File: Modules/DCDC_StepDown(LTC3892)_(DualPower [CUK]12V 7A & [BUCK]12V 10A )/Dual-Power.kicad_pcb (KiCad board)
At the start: 4 copper layers, 58.4 x 55.9 mm, 81 parts, among them J1 Conn_02x05_Top_Bottom, J2 Conn_02x05_Top_Bottom, J3 Conn_01x02, Q1 BSC028N06LS3, Q2 BSC028N06LS3, Q3 BSC028N06LS3, Q4 BSC028N06LS3, Q5 BSC028N06LS3, U1 LTC3892EUHPBF, U2 LT1797

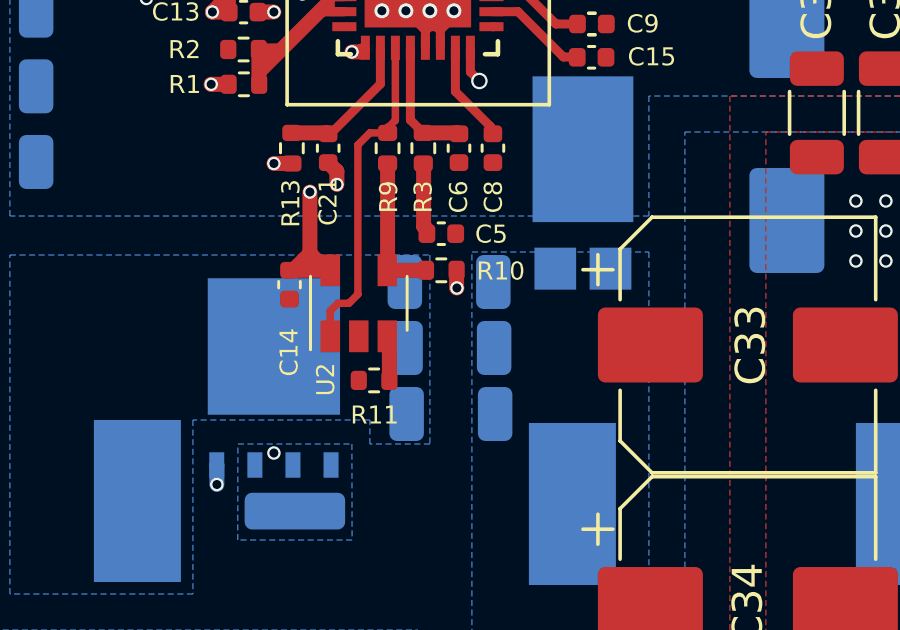
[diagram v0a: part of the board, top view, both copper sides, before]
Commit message: do rename
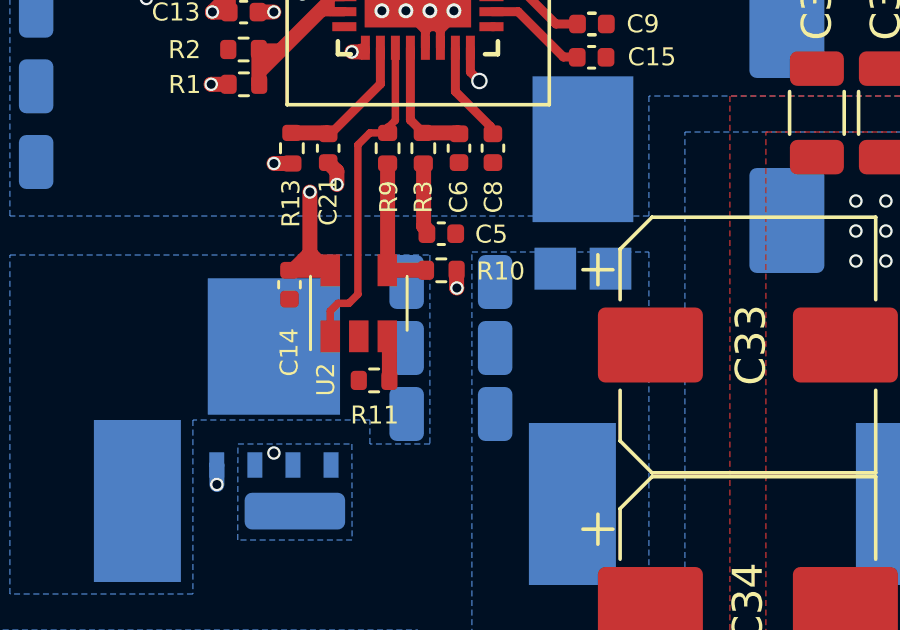
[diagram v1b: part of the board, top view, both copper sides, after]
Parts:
- moved C18 0.06 mm to (143.9, 97.6)
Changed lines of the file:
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@@
       (disableapertmacros false)
       (usegerberextensions false)
-      (usegerberattributes true)
+      (usegerberattributes false)
       (usegerberadvancedattributes true)
       (creategerberjobfile true)
@@
   )
   (footprint "Capacitor_SMD:C_1206_3216Metric" (layer "B.Cu")
-    (at 143.84 97.6 180)
+    (at 143.9 97.6 180)
     (descr "Capacitor SMD 1206 (3216 Metric), square (rectangular) end terminal, IPC_7351 nominal, (Body size source: IPC-SM-782 page 76, https://www.pcb-3d.com/wordpress/wp-content/uploads/ipc-sm-782a_amendment_1_and_2.pdf), generated with kicad-footprint-generator")
     (tags "capacitor")
@@
   )
   (footprint "Capacitor_SMD:C_1206_3216Metric" (layer "B.Cu")
-    (at 143.865 99.8 180)
+    (at 143.9 99.8 180)
     (descr "Capacitor SMD 1206 (3216 Metric), square (rectangular) end terminal, IPC_7351 nominal, (Body size source: IPC-SM-782 page 76, https://www.pcb-3d.com/wordpress/wp-content/uploads/ipc-sm-782a_amendment_1_and_2.pdf), generated with kicad-footprint-generator")
     (tags "capacitor")
